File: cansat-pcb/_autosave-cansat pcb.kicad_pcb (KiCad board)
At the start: 2 copper layers, 63 x 109 mm, 21 parts, among them J1 Conn_01x02_Pin, J4 Conn_01x03_Pin, J5 Conn_01x03_Pin, J6 Conn_01x03_Pin, Q1 AO3400A, Q2 2N3904, Q3 DMG2301L, SW1 SW_DPDT_x2, U3 MPU6050, U5 SGP30

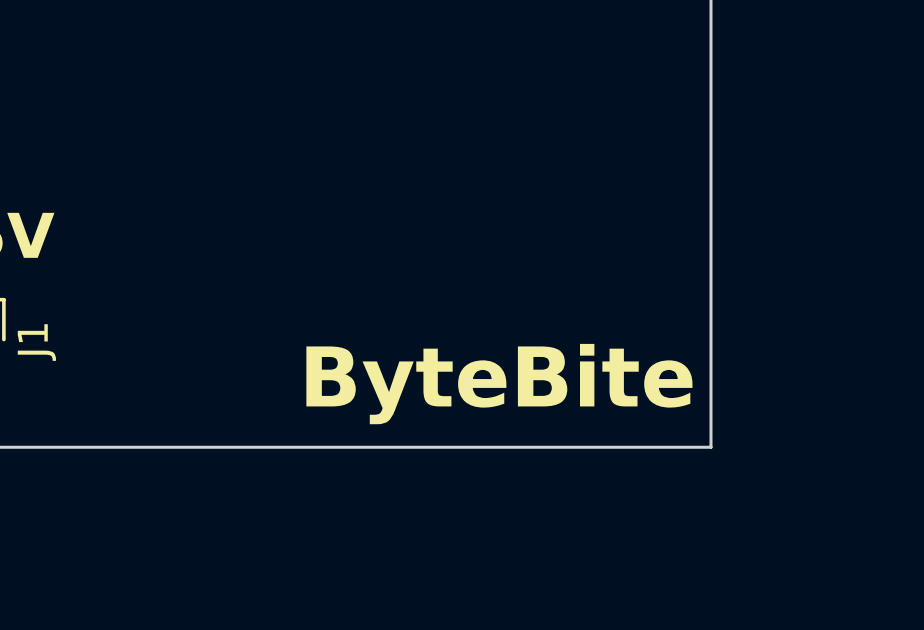
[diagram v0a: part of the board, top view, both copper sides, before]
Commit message: pcb V2
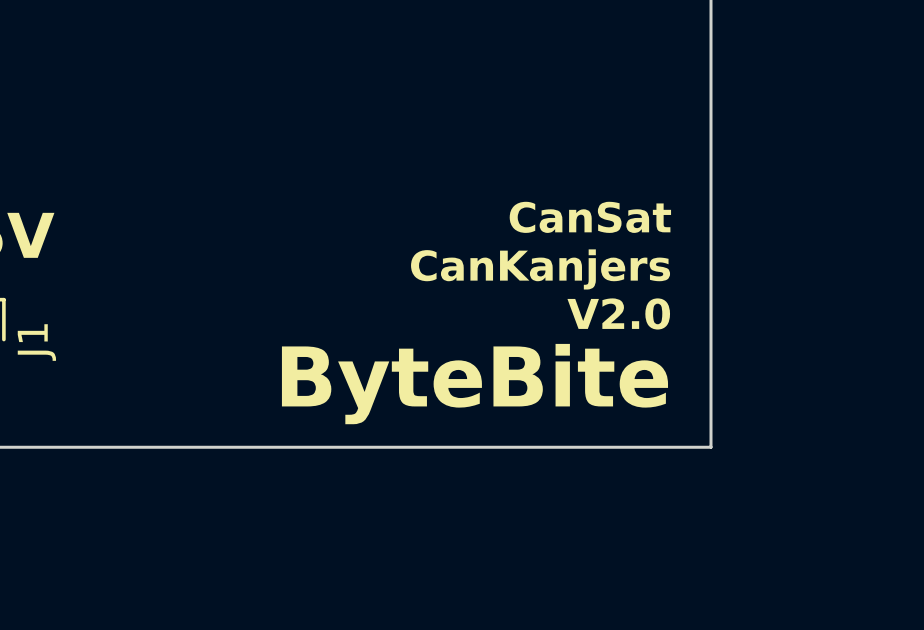
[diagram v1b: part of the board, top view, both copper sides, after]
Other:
- board text added: "CanSat CanKanjers V2.0"
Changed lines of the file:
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@@
   (setup
     (pad_to_mask_clearance 0)
-    (grid_origin 152.14 59.58)
+    (grid_origin 177.54 135.78)
     (pcbplotparams
       (layerselection 0x00010fc_ffffffff)
@@
     (effects (font (size 1.5 1.5) (thickness 0.3) bold) (justify left bottom))
   )
-  (gr_text "ByteBite" (at 181.888 146.714) (layer "F.SilkS")
-    (effects (font (size 2 2) (thickness 0.4) bold))
+  (gr_text "CanSat\nCanKanjers\nV2.0" (at 187.7 145.178) (layer "F.SilkS")
+    (effects (font (size 1 1) (thickness 0.2) bold) (justify right bottom))
+  )
+  (gr_text "ByteBite" (at 187.7 146.714) (layer "F.SilkS")
+    (effects (font (size 2 2) (thickness 0.4) bold) (justify right))
   )
   (segment (start 152.67 78.896) (end 156.006 78.896) (width 0.25) (layer "F.Cu") (net 1))
@@
     )
   )
+  (group "" (id 2326a1ff-ea58-45eb-ac90-ccae38486457)
+    (members
+      74ee758d-d28b-4c85-8a1d-747cfb82e51b
+      9ecb90c8-c273-47ff-8d79-826d2735b5df
+    )
+  )
